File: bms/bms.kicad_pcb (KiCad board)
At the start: 2 copper layers, 87.2 x 145.7 mm, 35 parts, among them J10 Conn_02x10_Odd_Even, J11 Conn_02x08_Odd_Even, J12 Conn_02x10_Odd_Even, J13 Conn_02x08_Odd_Even, J14 Conn_02x08_Odd_Even, J15 Conn_02x10_Odd_Even, J2 Conn_01x08_Socket, J3 Conn_01x06_Socket, J5 Conn_01x10_Socket, J6 Conn_01x08_Socket

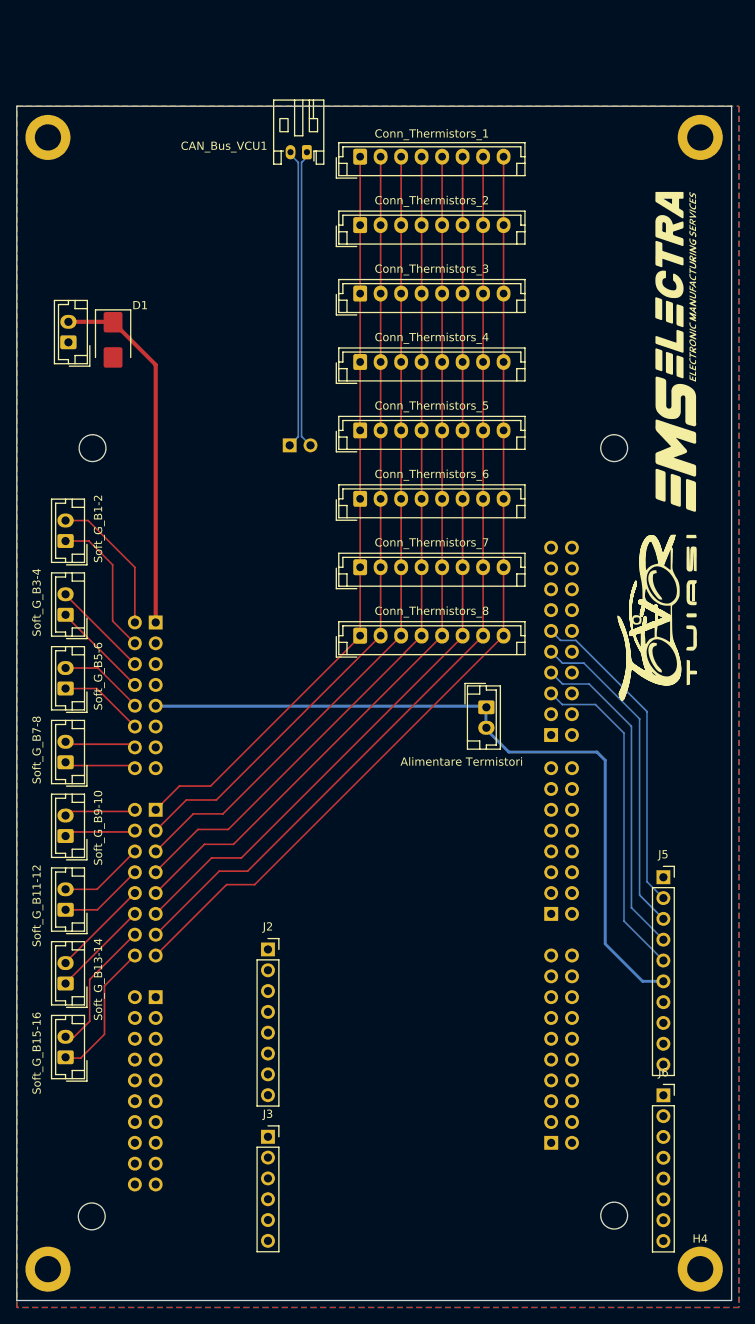
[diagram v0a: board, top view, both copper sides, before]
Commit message: added datasheets and revised layout to be continued
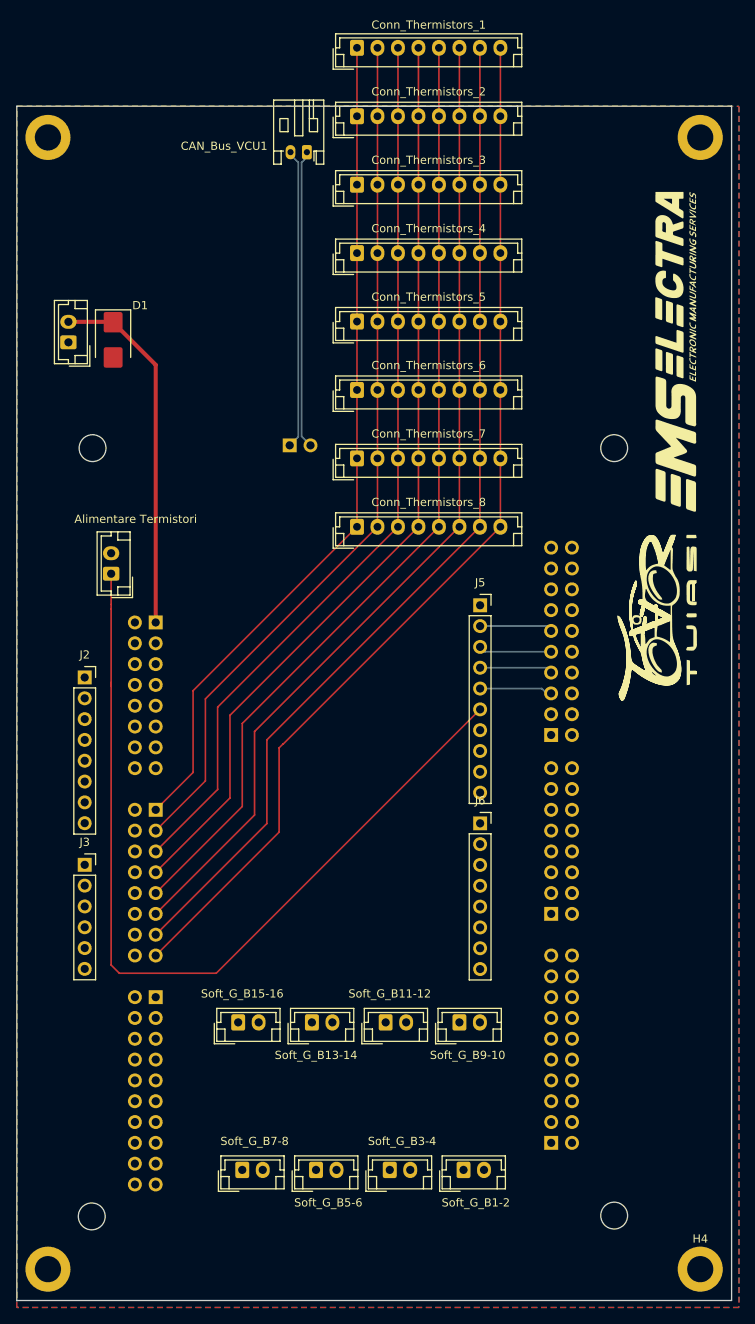
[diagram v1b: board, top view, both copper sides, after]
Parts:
- moved Soft_G_B1-2 90.8 mm to (102.0, 166.0), turned to 0 degrees
- moved Soft_G_B3-4 78.4 mm to (93.0, 166.0), turned to 0 degrees
- moved Soft_G_B5-6 66.2 mm to (84.0, 166.0), turned to 0 degrees
- moved Soft_G_B7-8 54.2 mm to (75.0, 166.0), turned to 0 degrees
- moved Soft_G_B9-10 53.2 mm to (101.5, 148.0), turned to 0 degrees
- moved Vdd1 48.6 mm to (59.0, 93.2), turned to 90 degrees
- moved Soft_G_B11-12 41.4 mm to (92.5, 148.0), turned to 0 degrees
- moved J2 40.0 mm to (55.8, 105.9)
- moved J5 40.0 mm to (104.0, 97.1)
- moved J6 40.0 mm to (104.0, 123.7)
- moved J3 40.0 mm to (55.8, 128.8)
- moved Soft_G_B13-14 30.4 mm to (83.5, 148.0), turned to 0 degrees
- moved Soft_G_B15-16 21.5 mm to (74.5, 148.0), turned to 0 degrees
- moved Conn_Thermistors_1 13.3 mm to (89.0, 87.5)
- moved Conn_Thermistors_3 13.3 mm to (89.0, 37.4)
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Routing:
- net SCK: track 40.6 -> 8.91 mm
- net MISO: track 40.2 -> 8.91 mm
- net SOUT: track 39.8 -> 8.91 mm
- net CS: track 39.4 -> 8.91 mm
- net G2: track 17.7 -> 0.00 mm
- net G1: track 17.6 -> 0.01 mm
- net G16: track 17.1 -> 0.00 mm
- net Vdd: track 90.5 -> 107.1 mm
- net G15: track 16.6 -> 0.05 mm
- net G4: track 12.1 -> 0.00 mm
- net G13: track 12.0 -> 0.00 mm
- net G3: track 12.0 -> 0.00 mm
- net G14: track 12.0 -> 0.00 mm
- net 8: track 117.1 -> 128.2 mm
- net 7: track 113.5 -> 124.6 mm
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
